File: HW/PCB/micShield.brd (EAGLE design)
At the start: 61.4 x 18.2 mm, 44 parts, among them M1 PMM-3738-VM1010-R, U1 LM27762DSSR, U2 LT6002CGN

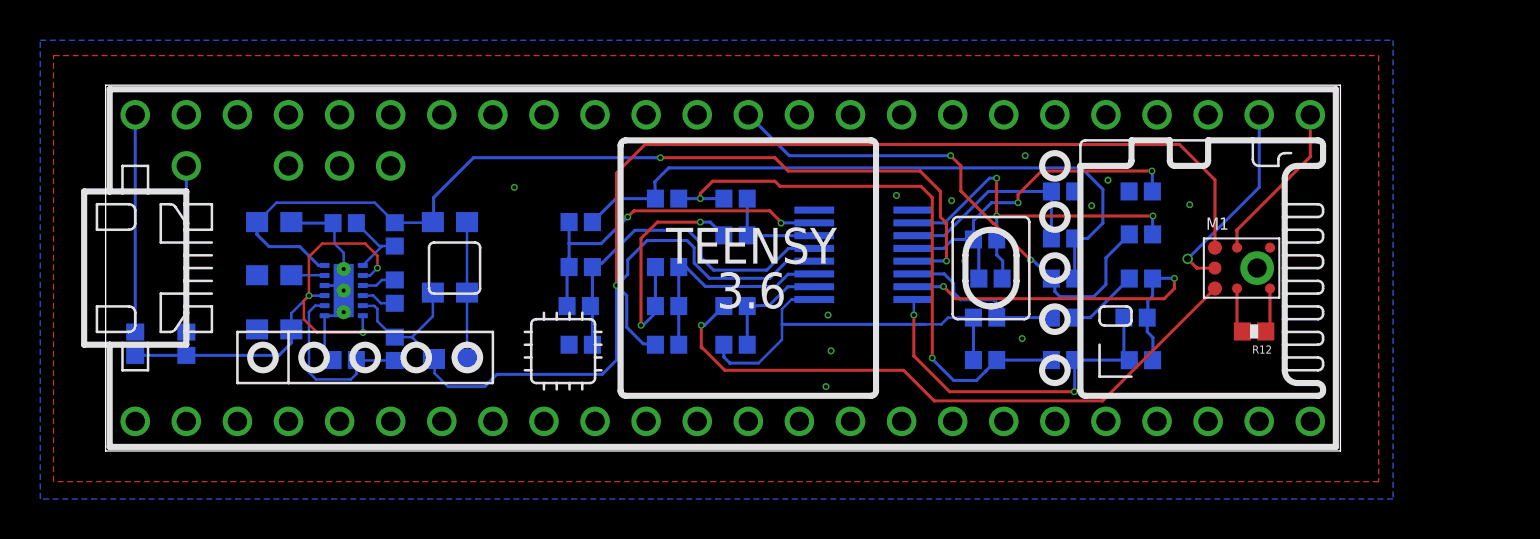
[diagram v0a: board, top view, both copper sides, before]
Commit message: Woohoo. Version 0.1 ordered.
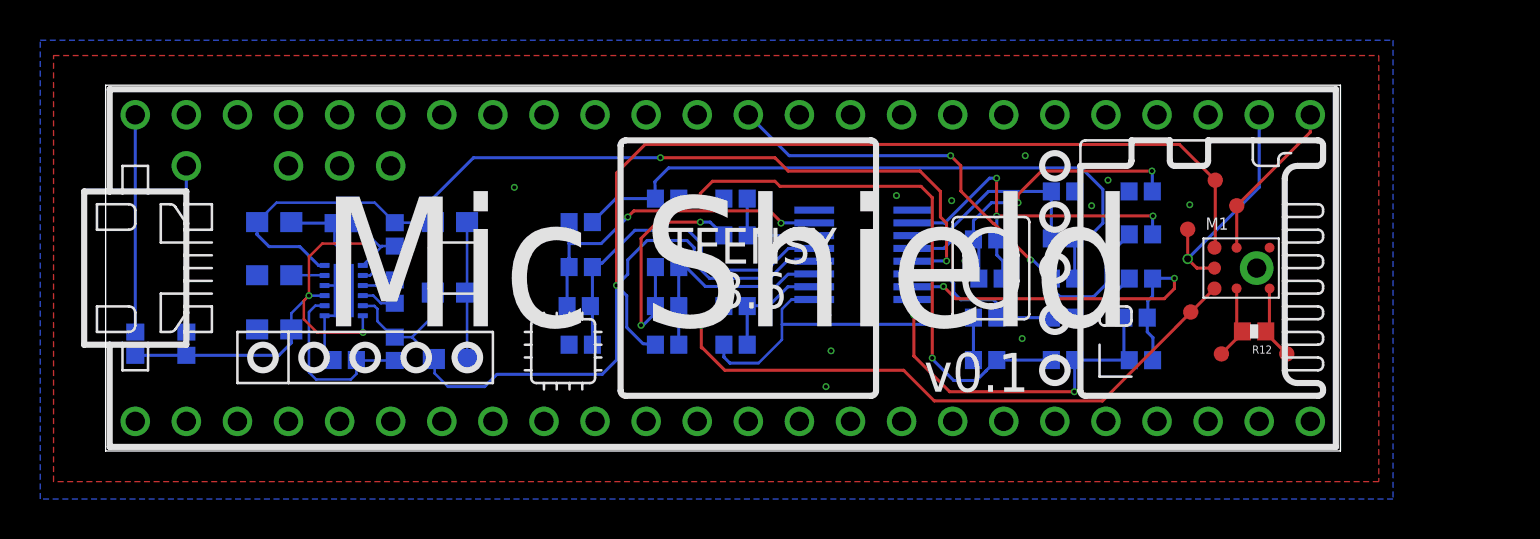
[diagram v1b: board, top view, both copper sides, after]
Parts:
- added FRAME1, FRAME2: FRAME-LETTER, SparkFun-Aesthetics:CREATIVE_COMMONS
- added TP1, TP2, TP3, TP4, TP5, TP6: TEST-POINT3, SparkFun-Passives:PAD.03X.03
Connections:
- net DOUT: now also TP6.P$1
- net GA1: now also TP3.P$1
- net GA2: now also TP2.P$1
- net MODE: now also TP4.P$1
- net TO_AMP: now also TP5.P$1
- net V3_3P: now also TP1.P$1
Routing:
- net GA1: track 2.22 -> 4.13 mm
- net GA2: track 2.25 -> 4.03 mm
- net DOUT: track 10.2 -> 11.6 mm
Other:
- board text added: "Mic Shield"
- board text added: "v0.1"
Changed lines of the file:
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@@
 <setting verticaltext="up"/>
 </settings>
-<grid distance="2" unitdist="mil" unit="mil" style="lines" multiple="1" display="no" altdistance="5" altunitdist="mil" altunit="mil"/>
+<grid distance="2" unitdist="mil" unit="mm" style="lines" multiple="1" display="no" altdistance="5" altunitdist="mil" altunit="mil"/>
 <layers>
 <layer number="1" name="Top" color="4" fill="1" visible="yes" active="yes"/>
@@
 <layer number="19" name="Unrouted" color="6" fill="1" visible="yes" active="yes"/>
 <layer number="20" name="Dimension" color="24" fill="1" visible="yes" active="yes"/>
-<layer number="21" name="tPlace" color="7" fill="1" visible="yes" active="yes"/>
+<layer number="21" name="tPlace" color="7" fill="1" visible="no" active="yes"/>
 <layer number="22" name="bPlace" color="7" fill="1" visible="yes" active="yes"/>
 <layer number="23" name="tOrigins" color="15" fill="1" visible="yes" active="yes"/>
@@
 <layer number="25" name="tNames" color="7" fill="1" visible="yes" active="yes"/>
 <layer number="26" name="bNames" color="7" fill="1" visible="yes" active="yes"/>
-<layer number="27" name="tValues" color="7" fill="1" visible="yes" active="yes"/>
+<layer number="27" name="tValues" color="7" fill="1" visible="no" active="yes"/>
 <layer number="28" name="bValues" color="7" fill="1" visible="yes" active="yes"/>
 <layer number="29" name="tStop" color="7" fill="3" visible="no" active="yes"/>
@@
 <layer number="42" name="bRestrict" color="1" fill="10" visible="yes" active="yes"/>
 <layer number="43" name="vRestrict" color="2" fill="10" visible="no" active="yes"/>
-<layer number="44" name="Drills" color="7" fill="1" visible="yes" active="yes"/>
+<layer number="44" name="Drills" color="7" fill="1" visible="no" active="yes"/>
 <layer number="45" name="Holes" color="7" fill="1" visible="yes" active="yes"/>
-<layer number="46" name="Milling" color="3" fill="1" visible="no" active="yes"/>
+<layer number="46" name="Milling" color="3" fill="1" visible="yes" active="yes"/>
 <layer number="47" name="Measures" color="7" fill="1" visible="no" active="yes"/>
 <layer number="48" name="Document" color="7" fill="1" visible="no" active="yes"/>
@@
 <wire x1="105.283" y1="31.242" x2="43.8912" y2="31.242" width="0" layer="20"/>
 <wire x1="43.8912" y1="31.242" x2="43.8912" y2="13.0556" width="0" layer="20"/>
+<text x="54.5592" y="19.2532" size="6.4516" layer="25">Mic Shield</text>
+<text x="84.582" y="16.002" size="1.9304" layer="25">v0.1</text>
 </plain>
 <attributes>
@@
 </class>
 </classes>
-<designrules name="jlcpcb-dru">
+<designrules name="jlcpcb-dru *">
 <description language="de">&lt;b&gt;EAGLE Design Rules&lt;/b&gt;
 &lt;p&gt;
@@
 <param name="mnLayersViaInSmd" value="2"/>
 <param name="mdCopperDimension" value="40mil"/>
-<param name="mdDrill" value="6mil"/>
+<param name="mdDrill" value="8mil"/>
 <param name="mdSmdStop" value="0mil"/>
 <param name="msWidth" value="5mil"/>
@@
 <attribute name="NAME" x="96.7611" y="22.23756875" size="0.4064" layer="26" font="vector" rot="MR180"/>
 </element>
-<element name="M1" library="MIC" package="PMM-3738-VM1010-R" value="PMM-3738-VM1010-R" x="101.1428" y="22.1488" rot="MR0"/>
+<element name="M1" library="MIC" package="PMM-3738-VM1010-R" value="PMM-3738-VM1010-R" x="101.12" y="22.1488" rot="MR0"/>
 <element name="R15" library="SparkFun-Resistors" package="0402-RES" value="" x="71.8058" y="18.3388" rot="MR180"/>
 <element name="R16" library="SparkFun-Resistors" package="0402-RES" value="" x="71.8058" y="20.259675" rot="MR0"/>
@@
 <element name="R10" library="SparkFun-Resistors" package="0402-RES" value="" x="45.3644" y="18.3896" rot="MR90"/>
 <element name="R12" library="SparkFun-Resistors" package="0402-RES" value="" x="100.9904" y="18.9992" rot="R180"/>
+<element name="FRAME2" library="SparkFun-Aesthetics" package="CREATIVE_COMMONS" value="FRAME-LETTER" x="36.9824" y="6.1468"/>
+<element name="FRAME1" library="SparkFun-Aesthetics" package="CREATIVE_COMMONS" value="FRAME-LETTER" x="35.9664" y="5.1308"/>
+<element name="TP1" library="SparkFun-Passives" package="PAD.03X.03" value="TEST-POINT3" x="99.06" y="26.5176"/>
+<element name="TP2" library="SparkFun-Passives" package="PAD.03X.03" value="TEST-POINT3" x="99.3648" y="17.8816"/>
+<element name="TP3" library="SparkFun-Passives" package="PAD.03X.03" value="TEST-POINT3" x="102.616" y="17.8816"/>
+<element name="TP4" library="SparkFun-Passives" package="PAD.03X.03" value="TEST-POINT3" x="100.1268" y="25.2476"/>
+<element name="TP5" library="SparkFun-Passives" package="PAD.03X.03" value="TEST-POINT3" x="97.8408" y="19.9644"/>
+<element name="TP6" library="SparkFun-Passives" package="PAD.03X.03" value="TEST-POINT3" x="97.6884" y="24.0792"/>
 </elements>
 <signals>
@@
 <contactref element="R1" pad="1"/>
 <contactref element="M1" pad="1"/>
-<wire x1="99.0428" y1="21.1338" x2="93.4538" y2="15.5448" width="0.1524" layer="1"/>
+<wire x1="99.02" y1="21.1338" x2="93.4538" y2="15.5448" width="0.1524" layer="1"/>
 <via x="73.5076" y="19.304" extent="1-16" drill="0.2"/>
 <wire x1="73.5076" y1="19.304" x2="73.673725" y2="19.304" width="0.1524" layer="16"/>
@@
 <wire x1="73.5076" y1="18.1864" x2="73.5584" y2="18.1864" width="0.1524" layer="1"/>
 <wire x1="73.5584" y1="18.1864" x2="74.676" y2="17.0688" width="0.1524" layer="1"/>
+<contactref element="TP5" pad="P$1"/>
+<wire x1="99.02" y1="21.1338" x2="97.8408" y2="19.9644" width="0" layer="19" extent="1-1"/>
 </signal>
 <signal name="MODE">
 <contactref element="M1" pad="5"/>
 <contactref element="U$1" pad="33/A14"/>
-<wire x1="100.1428" y1="23.1638" x2="100.1428" y2="24.0124" width="0.1524" layer="1"/>
-<wire x1="100.1428" y1="24.0124" x2="100.1268" y2="24.0284" width="0.1524" layer="1"/>
-<wire x1="100.1268" y1="24.0284" x2="103.7844" y2="27.686" width="0.1524" layer="1"/>
-<wire x1="103.7844" y1="27.686" x2="103.7844" y2="29.7688" width="0.1524" layer="1"/>
+<wire x1="100.12" y1="23.1638" x2="100.1268" y2="23.1706" width="0.1524" layer="1"/>
+<wire x1="100.1268" y1="23.1706" x2="100.1268" y2="25.2476" width="0.1524" layer="1"/>
+<wire x1="100.1268" y1="25.2476" x2="103.7844" y2="28.9052" width="0.1524" layer="1"/>
+<wire x1="103.7844" y1="28.9052" x2="103.7844" y2="29.7688" width="0.1524" layer="1"/>
+<contactref element="TP4" pad="P$1"/>
 </signal>
 <signal name="GA1">
 <contactref element="M1" pad="3"/>
 <contactref element="R12" pad="1"/>
-<wire x1="101.7828" y1="21.1338" x2="101.7828" y2="19.2116" width="0.1524" layer="1"/>
+<wire x1="101.76" y1="21.1338" x2="101.7524" y2="21.1262" width="0.1524" layer="1"/>
+<wire x1="101.7524" y1="21.1262" x2="101.7524" y2="18.9992" width="0.1524" layer="1"/>
+<wire x1="101.7524" y1="18.9992" x2="101.7828" y2="19.2116" width="0.1524" layer="1"/>
 <wire x1="101.7828" y1="19.2116" x2="101.5704" y2="18.9992" width="0.1524" layer="1"/>
+<contactref element="TP3" pad="P$1"/>
+<wire x1="102.616" y1="17.8816" x2="101.7524" y2="18.7452" width="0.1524" layer="1"/>
+<wire x1="101.7524" y1="18.7452" x2="101.7524" y2="18.9992" width="0.1524" layer="1"/>
 </signal>
 <signal name="GA2">
 <contactref element="M1" pad="2"/>
 <contactref element="R12" pad="2"/>
-<wire x1="100.1428" y1="21.1338" x2="100.1428" y2="19.2668" width="0.1524" layer="1"/>
+<wire x1="100.12" y1="21.1338" x2="100.1268" y2="21.127" width="0.1524" layer="1"/>
+<wire x1="100.1268" y1="21.127" x2="100.1268" y2="19.1516" width="0.1524" layer="1"/>
+<wire x1="100.1268" y1="19.1516" x2="100.1428" y2="19.2668" width="0.1524" layer="1"/>
 <wire x1="100.1428" y1="19.2668" x2="100.4104" y2="18.9992" width="0.1524" layer="1"/>
+<contactref element="TP2" pad="P$1"/>
+<wire x1="99.3648" y1="17.8816" x2="100.4104" y2="18.9272" width="0.1524" layer="1"/>
+<wire x1="100.4104" y1="18.9272" x2="100.4104" y2="18.9992" width="0.1524" layer="1"/>
 </signal>
 <signal name="V3_3P">
@@
 <wire x1="60.2488" y1="17.5904" x2="60.2488" y2="16.9164" width="0.127" layer="16"/>
 <wire x1="60.9092" y1="16.256" x2="60.2488" y2="16.9164" width="0.127" layer="16"/>
-<wire x1="99.0428" y1="23.1638" x2="99.0428" y2="26.5348" width="0.1524" layer="1"/>
-<wire x1="99.0428" y1="26.5348" x2="97.282" y2="28.2956" width="0.1524" layer="1"/>
+<wire x1="99.02" y1="23.1638" x2="99.06" y2="23.1648" width="0.1524" layer="1"/>
+<wire x1="99.06" y1="23.1648" x2="99.06" y2="26.5176" width="0.1524" layer="1"/>
+<wire x1="99.06" y1="26.5176" x2="97.282" y2="28.2956" width="0.1524" layer="1"/>
 <wire x1="70.7136" y1="28.2956" x2="69.2912" y2="26.8732" width="0.1524" layer="1"/>
 <wire x1="97.282" y1="28.2956" x2="70.7136" y2="28.2956" width="0.1524" layer="1"/>
@@
 <wire x1="69.85" y1="22.5552" x2="69.85" y2="21.844" width="0.1524" layer="16"/>
 <wire x1="69.85" y1="21.844" x2="69.2912" y2="21.2852" width="0.1524" layer="16"/>
+<contactref element="TP1" pad="P$1"/>
 </signal>
 <signal name="DOUT">
 <contactref element="M1" pad="7"/>
 <contactref element="U$1" pad="34/A15"/>
-<wire x1="99.0428" y1="22.1488" x2="98.1456" y2="22.1488" width="0.1524" layer="1"/>
+<wire x1="99.02" y1="22.1488" x2="98.1456" y2="22.1488" width="0.1524" layer="1"/>
 <wire x1="98.1456" y1="22.1488" x2="97.6884" y2="22.606" width="0.1524" layer="1"/>
 <via x="97.6884" y="22.606" extent="1-16" drill="0.35"/>
 <wire x1="97.6884" y1="22.606" x2="101.2444" y2="26.162" width="0.1524" layer="16"/>
 <wire x1="101.2444" y1="26.162" x2="101.2444" y2="29.7688" width="0.1524" layer="16"/>
+<contactref element="TP6" pad="P$1"/>
+<wire x1="97.6884" y1="24.0792" x2="97.6884" y2="22.606" width="0.1524" layer="1"/>
 </signal>
 <signal name="N$6">
